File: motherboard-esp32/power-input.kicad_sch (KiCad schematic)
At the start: 13 parts, among them J3 JST_2P_XH, Q1 DOD4185, Q2 DOD4185

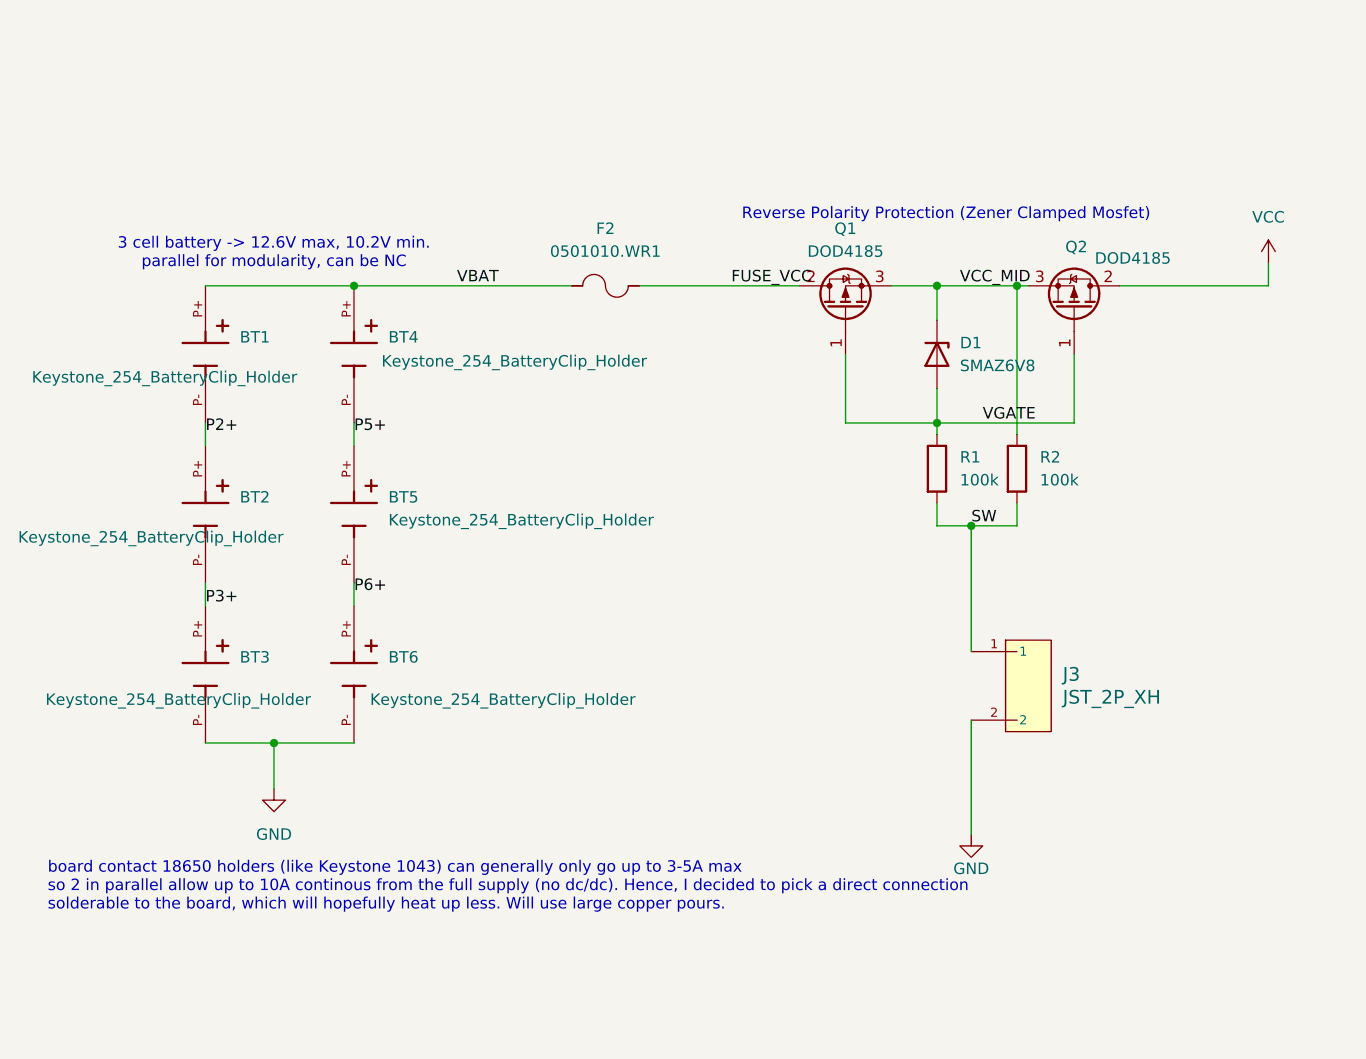
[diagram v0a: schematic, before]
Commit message: update
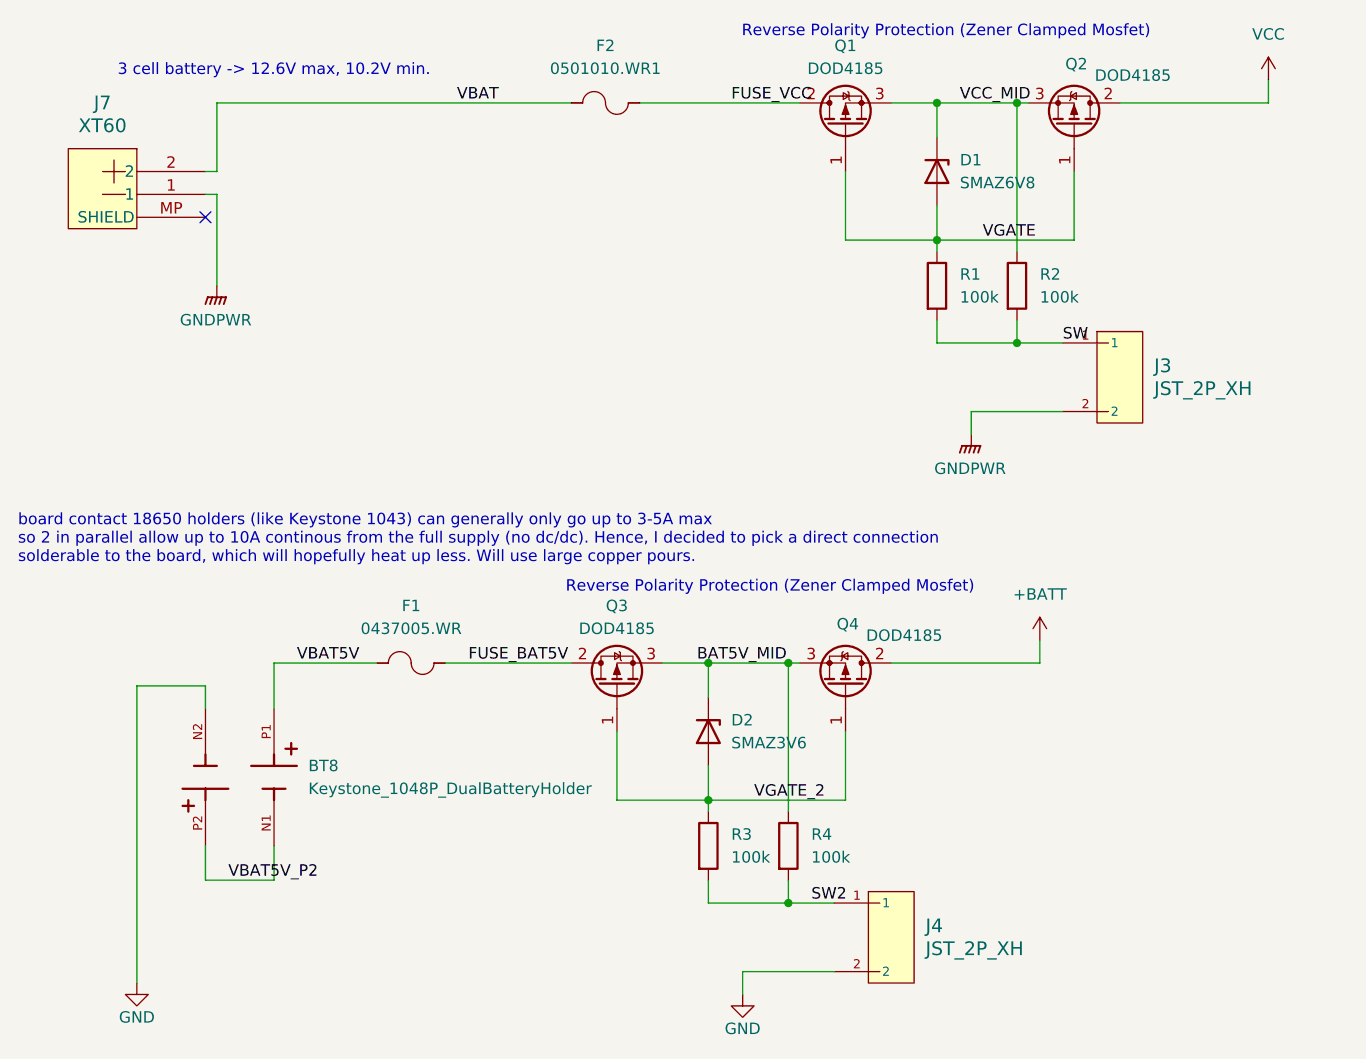
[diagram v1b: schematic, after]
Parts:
- removed BT1, BT2, BT3, BT4, BT5, BT6: Keystone_254_BatteryClip_Holder, bio-robot:BAT_254_18650_Holder, symbol bio-robot:Keystone_254_BatteryClip_Holder
- added BT8: Keystone_1048P_DualBatteryHolder, bio-robot:BAT_1048P, symbol bio-robot:Keystone_1048P_DualBatteryHolder
- added D2: SMAZ3V6, bots:D_SMA, symbol bio-robot:D_ZENER_SMAZ3V6
- added F1: 0437005.WR, bio-robot:Fuse_1206_3216Metric, symbol bio-robot:Fuse_0437005.WR
- added J4: JST_2P_XH, bio-robot:JST_B2B-XH-A_LF__SN_, symbol bio-robot:JST_XH-2
- added J7: XT60, bio-robot:AMASS_XT60PW-M, symbol bio-robot:XT-60-RA
- added Q3, Q4: DOD4185, bio-robot:DPAK-3_ONS, symbol bio-robot:Q_Pch40V45A
- added R3, R4: 100k, bio-robot:R_0603_1608Metric, symbol bio-robot:R_100k
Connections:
- net GND: now also BT8.N2, J4.2; no longer J3.2
- net VBAT: now also J7.2
- new net +BATT: Q4.2 (D)
- new net BAT5V_MID: D2.1 (K), Q3.3 (S), Q4.3 (S), R4.1
- new net FUSE_BAT5V: F1.2, Q3.2 (D)
- new net GNDPWR: J3.2, J7.1
- new net SW2: J4.1, R3.2, R4.2
- new net VBAT5V: BT8.P1, F1.1
- new net VBAT5V_P2: BT8.N1, BT8.P2
- new net VGATE_2: D2.2 (A), Q3.1 (G), Q4.1 (G), R3.1
- no-connect marks 0 -> 1
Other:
- note added: "3 cell battery -> 12.6V max, 10.2V min."
- note removed: "3 cell battery -> 12.6V max, 10.2V min. parallel for modularity, can be NC"
- moved on the sheet: D1, F2, J3, Q1, Q2, R1, R2

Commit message: update
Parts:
- D1: footprint bio-robot:D_SMA -> bots:D_SMA
- J3, J4: footprint bio-robot:JST_B2B-XH-A_LF__SN_ -> bots:JST_B2B-XH-A_LF__SN_
- Q1, Q2, Q3, Q4: footprint bio-robot:DPAK-3_ONS -> bots:DPAK-3_ONS
- R1, R2, R3, R4: footprint bio-robot:R_0603_1608Metric -> bots:R_0603_1608Metric
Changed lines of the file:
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@@
 			)
 		)
-		(property "Footprint" "bio-robot:JST_B2B-XH-A_LF__SN_"
+		(property "Footprint" "bots:JST_B2B-XH-A_LF__SN_"
 			(at 116.84 107.95 0)
 			(hide yes)
@@
 			)
 		)
-		(property "Footprint" "bio-robot:R_0603_1608Metric"
+		(property "Footprint" "bots:R_0603_1608Metric"
 			(at 104.902 111.76 90)
 			(hide yes)
@@
 			)
 		)
-		(property "Footprint" "bio-robot:DPAK-3_ONS"
+		(property "Footprint" "bots:DPAK-3_ONS"
 			(at 111.125 89.027 0)
 			(hide yes)
@@
 			)
 		)
-		(property "Footprint" "bio-robot:R_0603_1608Metric"
+		(property "Footprint" "bots:R_0603_1608Metric"
 			(at 121.412 49.53 90)
 			(hide yes)
@@
 			)
 		)
-		(property "Footprint" "bio-robot:D_SMA"
+		(property "Footprint" "bots:D_SMA"
 			(at 123.19 36.83 0)
 			(hide yes)
@@
 			)
 		)
-		(property "Footprint" "bio-robot:R_0603_1608Metric"
+		(property "Footprint" "bots:R_0603_1608Metric"
 			(at 96.012 111.76 90)
 			(hide yes)
@@
 			)
 		)
-		(property "Footprint" "bio-robot:DPAK-3_ONS"
+		(property "Footprint" "bots:DPAK-3_ONS"
 			(at 136.525 26.797 0)
 			(hide yes)
@@
 			)
 		)
-		(property "Footprint" "bio-robot:DPAK-3_ONS"
+		(property "Footprint" "bots:DPAK-3_ONS"
 			(at 114.935 26.797 0)
 			(hide yes)
@@
 			)
 		)
-		(property "Footprint" "bio-robot:DPAK-3_ONS"
+		(property "Footprint" "bots:DPAK-3_ONS"
 			(at 89.535 89.027 0)
 			(hide yes)
@@
 			)
 		)
-		(property "Footprint" "bio-robot:R_0603_1608Metric"
+		(property "Footprint" "bots:R_0603_1608Metric"
 			(at 130.302 49.53 90)
 			(hide yes)
@@
 			)
 		)
-		(property "Footprint" "bio-robot:JST_B2B-XH-A_LF__SN_"
+		(property "Footprint" "bots:JST_B2B-XH-A_LF__SN_"
 			(at 142.24 45.72 0)
 			(hide yes)
